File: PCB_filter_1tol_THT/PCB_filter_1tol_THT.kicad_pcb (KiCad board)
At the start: 2 copper layers, 26 parts, among them J1 Conn_01x03_Pin, J2 Conn_01x02_Pin, U1 AD620, U2 LM2902N/NOPB

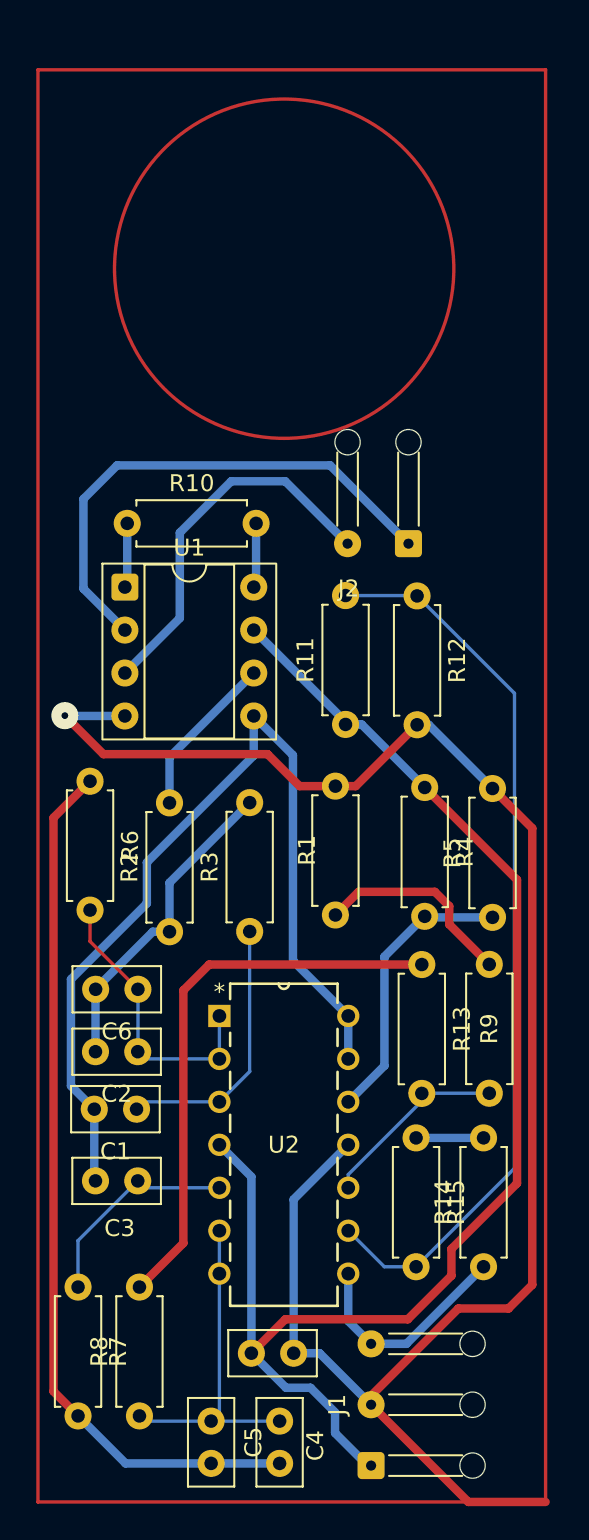
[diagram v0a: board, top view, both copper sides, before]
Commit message: last
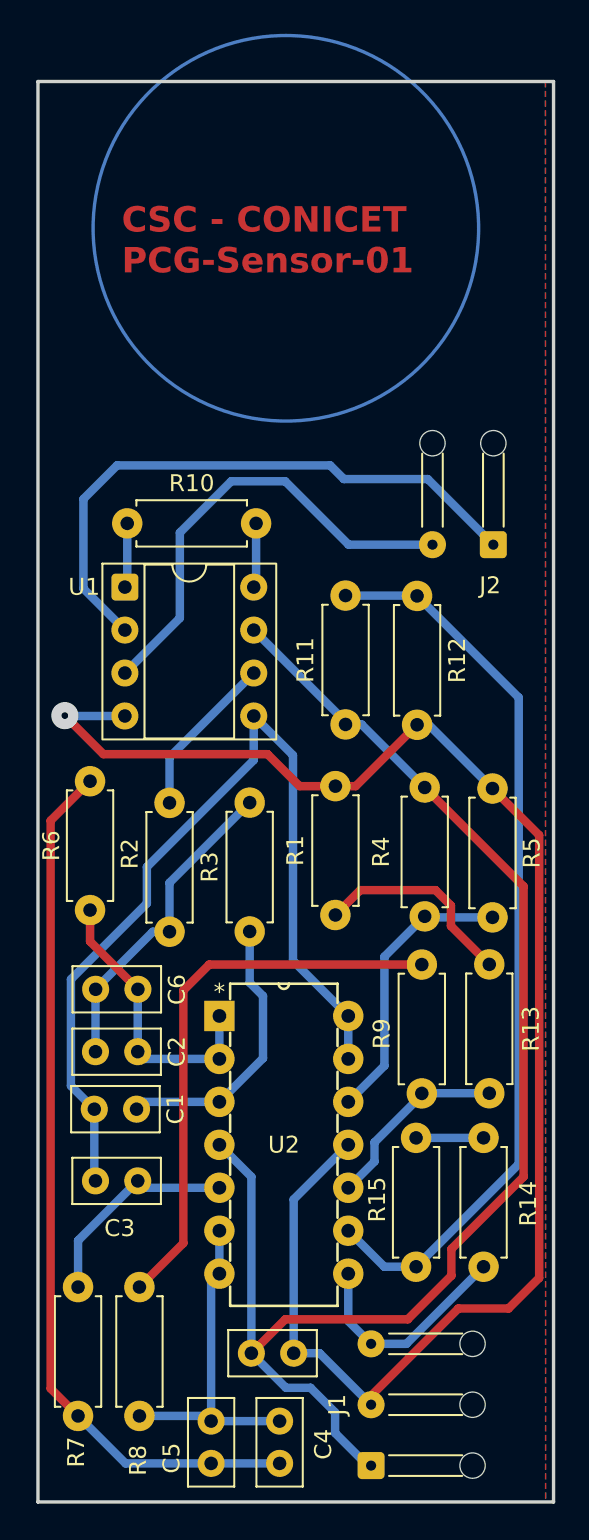
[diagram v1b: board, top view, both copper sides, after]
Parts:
- R1, R10, R11, R12, R13, R14, R15, R2, R3, R4, R5, R6, R7, R8, R9: footprint Resistor_THT:R_Axial_DIN0207_L6.3mm_D2.5mm_P7.62mm_Horizontal -> DAVID:R_hueco_grande
- moved J2 5.02 mm to (164.2, 77.8)
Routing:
- net GND: track 109.2 -> 96.8 mm
- net Net-(J2-Pin_2): track 22.4 -> 27.4 mm
- net Net-(J2-Pin_1): track 30.7 -> 35.8 mm
- net IN1+: track 15.9 -> 16.5 mm
- added copper zone on B.Cu, net GND
- added copper zone on F.Cu, net GND
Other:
- board outline added: 30.5 x 84 mm
- board text added: "CSC - CONICET PCG-Sensor-01"
